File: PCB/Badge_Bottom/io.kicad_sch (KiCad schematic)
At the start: 29 parts, among them CN1 JACK_OUT, CN2 JACK_IN, J1 USB_FS, J11 Power, J12 GPIO, J13 GPIO, J14 GPIO, J15 GPIO, J16 GPIO, J17 GPIO, J18 SAO, J19 Power, J2 USB_HS, SW1 TM-2024A, SW2 TM-2024A

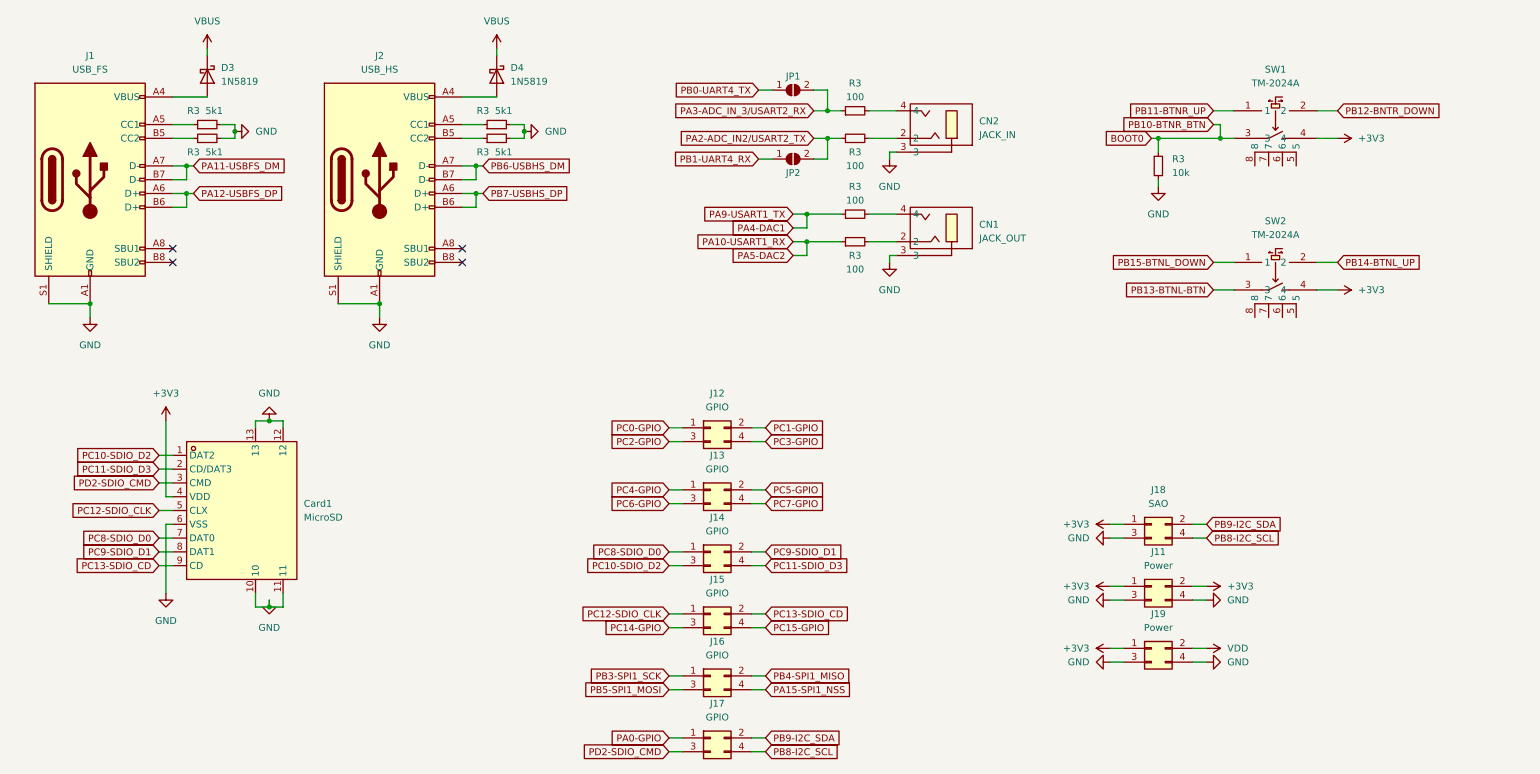
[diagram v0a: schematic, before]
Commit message: finised pcb layout
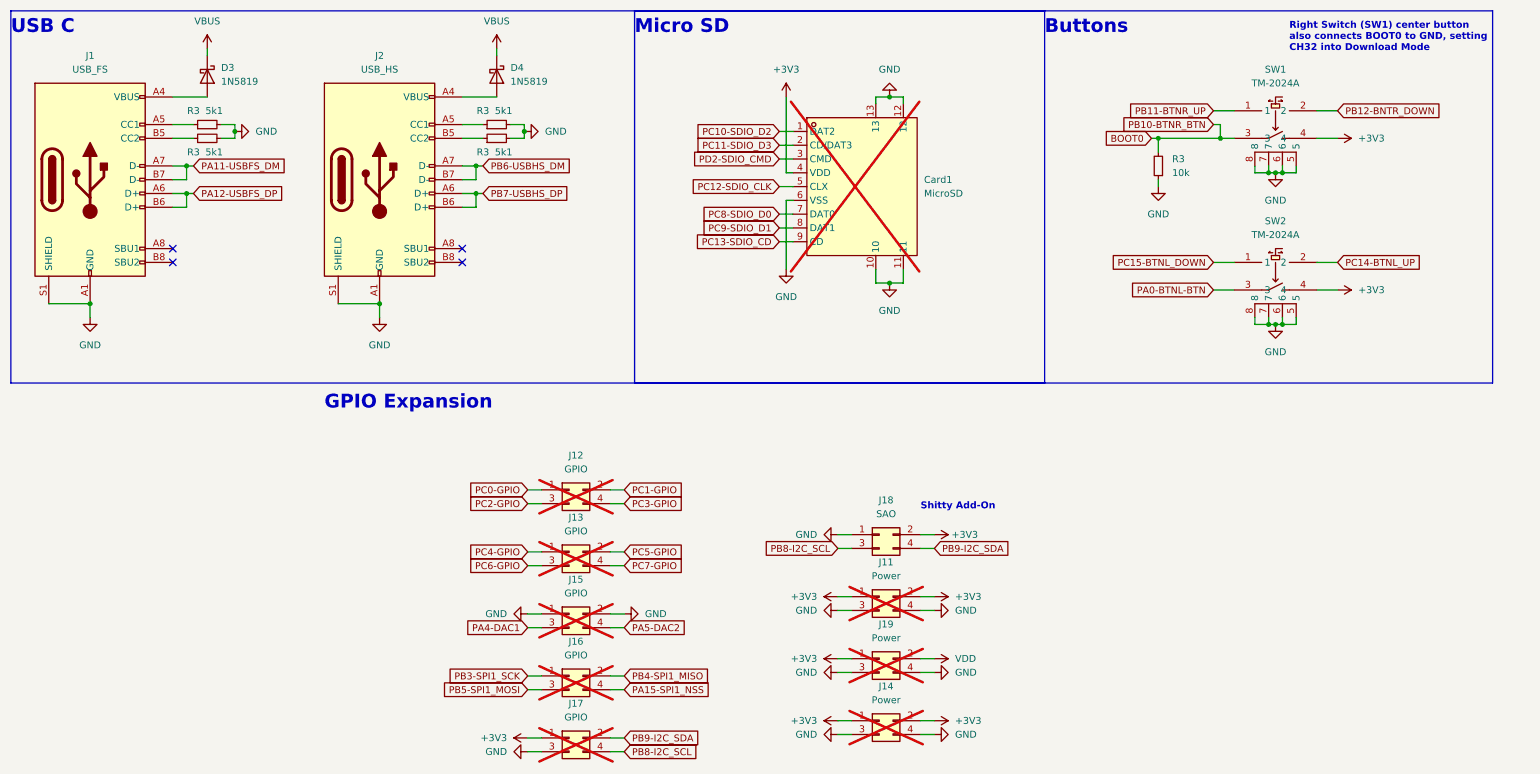
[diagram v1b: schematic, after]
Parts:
- removed CN1: JACK_OUT, PJ-320:AUDIO-TH_HOOYA_PJ-320, symbol PJ-320:PJ-320
- removed CN2: JACK_IN, PJ-320:AUDIO-TH_HOOYA_PJ-320, symbol PJ-320:PJ-320
- removed JP1, JP2: SolderJumper_2_Open, Jumper:SolderJumper-2_P1.3mm_Open_RoundedPad1.0x1.5mm, symbol Jumper:SolderJumper_2_Open
- removed R3 (x4): 100, Resistor_SMD:R_0603_1608Metric, symbol Device:R_Small
- Card1, J11, J12, J13, J15, J16, J17, J19: now not fitted
- J14: value GPIO -> Power; now not fitted
- J18: footprint Connector_PinSocket_2.54mm:PinSocket_2x02_P2.54mm_Horizontal -> 2x02_pinsocket_254:HDR-TH_4P-P2.54-H-F-R2-C2-W8.5
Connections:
- net PA0-GPIO is gone; now on net +3V3: J17.1 (Pin_1)
- net PC14-GPIO is gone; now on net PA4-DAC1: J15.3 (Pin_3)
- net +3V3: now also J14.1 (Pin_1), J14.2 (Pin_2), J18.2 (Pin_2); no longer J18.1 (Pin_1)
- net GND: now also J14.3 (Pin_3), J14.4 (Pin_4), J15.1 (Pin_1), J15.2 (Pin_2), J17.3 (Pin_3), J18.1 (Pin_1), SW1.5, SW1.6, SW1.7, SW1.8, SW2.5, SW2.6, SW2.7, SW2.8; no longer J18.3 (Pin_3)
- net PB8-I2C_SCL: now also J18.3 (Pin_3); no longer J18.4 (Pin_4)
- net PB9-I2C_SDA: now also J18.4 (Pin_4); no longer J18.2 (Pin_2)
- net PC10-SDIO_D2: no longer J14.3 (Pin_3)
- net PC11-SDIO_D3: no longer J14.4 (Pin_4)
- net PC12-SDIO_CLK: no longer J15.1 (Pin_1)
- net PC13-SDIO_CD: no longer J15.2 (Pin_2)
- net PC8-SDIO_D0: no longer J14.1 (Pin_1)
- net PC9-SDIO_D1: no longer J14.2 (Pin_2)
- net PD2-SDIO_CMD: no longer J17.3 (Pin_3)
- net PB13-BTNL-BTN renamed PA0-BTNL-BTN
- net PB14-BTNL_UP renamed PC14-BTNL_UP
- net PB15-BTNL_DOWN renamed PC15-BTNL_DOWN
- net PC15-GPIO renamed PA5-DAC2
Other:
- note added: "Buttons"
- note added: "GPIO Expansion"
- note added: "Micro SD"
- note added: "Right Switch (SW1) center button also connects BOOT0 to GND, setting CH32 into Download Mode"
- note added: "Shitty Add-On"
- note added: "USB C"
- moved on the sheet: J18
